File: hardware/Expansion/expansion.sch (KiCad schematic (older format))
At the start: 25 parts, among them J1 VID, J2 PPI, J3 PPO, P1 EXI, P2 EXO, U1 74LS138, U2 74LS00, U3 74LS123, U4 74LS20, U5 74LS175, U6 74LS245

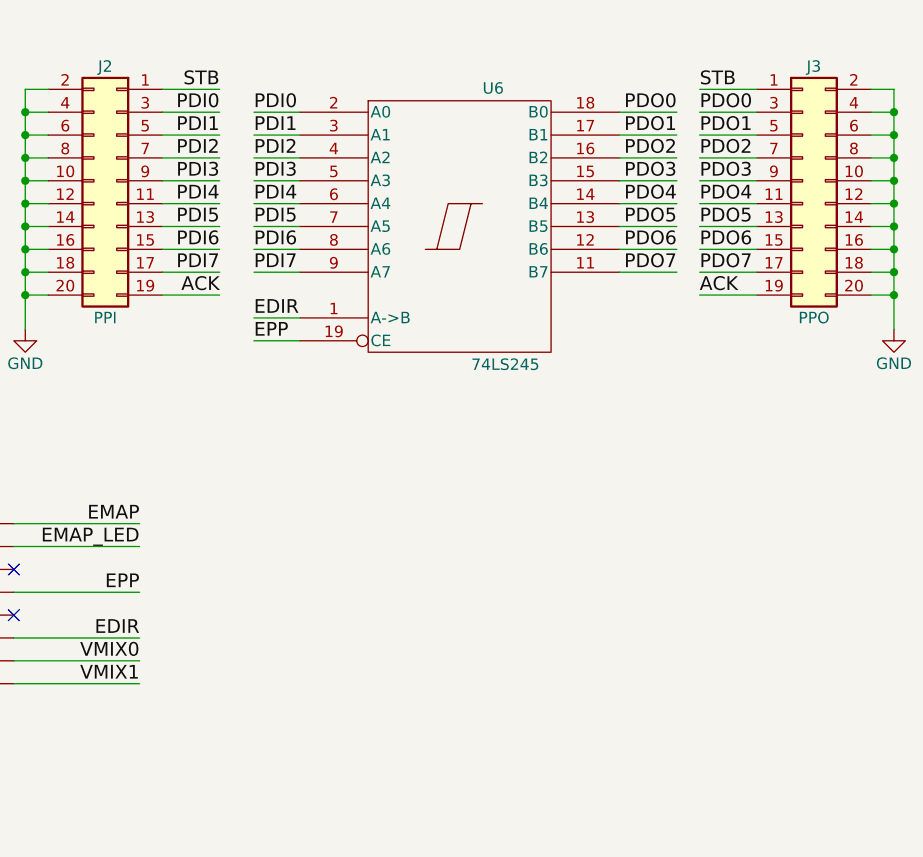
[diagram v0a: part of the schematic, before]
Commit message: revert:expansion
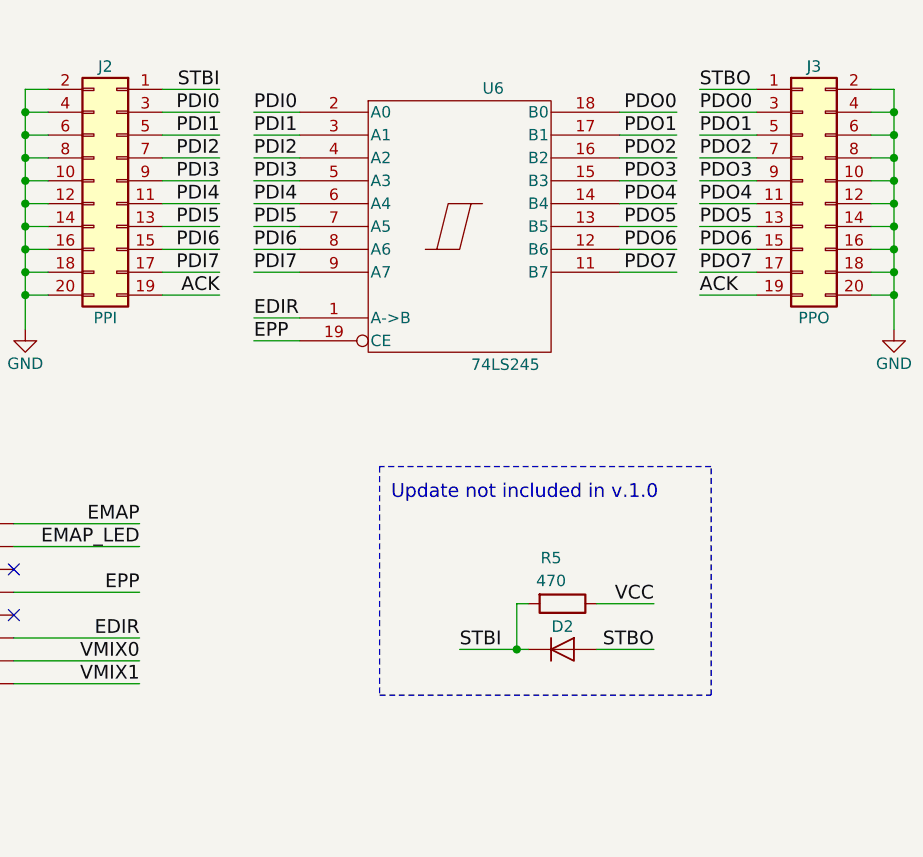
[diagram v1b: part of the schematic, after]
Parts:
- added D2: D, Diodes_THT:D_A-405_P7.62mm_Horizontal, symbol D
- added R5: 470, Resistors_THT:R_Axial_DIN0204_L3.6mm_D1.6mm_P7.62mm_Horizontal, symbol R
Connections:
- net VCC: now also R5.1
- net STB renamed STBI
- net STBI: now also D2.1 (K), R5.2; no longer J3.1 (Pin_1)
- new net STBO: D2.2 (A), J3.1 (Pin_1)
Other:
- note added: "Update not included in v.1.0"
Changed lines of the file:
@@
 Title "OricExos expansion board"
 Date "2018-11-30"
-Rev "1.0"
+Rev "1.1"
 Comp "copyright © 2018 iss"
 Comment1 ""
@@
 	7800 950  8050 950
 Text Label 8050 950  2    60   ~ 0
-STB
+STBI
 Wire Wire Line
 	10400 950  10150 950
 Text Label 10150 950  0    60   ~ 0
-STB
+STBO
 Wire Wire Line
 	10400 1850 10150 1850
@@
 	2550 3300 2550 4050
 Connection ~ 2550 4050
+$Comp
+L D D2
+U 1 1 5C12C7AE
+P 9550 3400
+F 0 "D2" H 9550 3500 50  0000 C CNN
+F 1 "D" H 9550 3300 50  0001 C CNN
+F 2 "Diodes_THT:D_A-405_P7.62mm_Horizontal" H 9550 3400 50  0001 C CNN
+F 3 "" H 9550 3400 50  0001 C CNN
+	1    9550 3400
+	1    0    0    -1
+$EndComp
+Wire Wire Line
+	9400 3400 9100 3400
+Text Label 9100 3400 0    60   ~ 0
+STBI
+Wire Wire Line
+	9700 3400 9950 3400
+Text Label 9950 3400 2    60   ~ 0
+STBO
+$Comp
+L R R5
+U 1 1 5C12D242
+P 9550 3200
+F 0 "R5" V 9350 3150 50  0000 C CNN
+F 1 "470" V 9450 3150 50  0000 C CNN
+F 2 "Resistors_THT:R_Axial_DIN0204_L3.6mm_D1.6mm_P7.62mm_Horizontal" V 9480 3200 50  0001 C CNN
+F 3 "" H 9550 3200 50  0001 C CNN
+	1    9550 3200
+	0    1    1    0
+$EndComp
+Wire Wire Line
+	9700 3200 9950 3200
+Text Label 9950 3200 2    60   ~ 0
+VCC
+Wire Wire Line
+	9400 3200 9350 3200
+Wire Wire Line
+	9350 3200 9350 3400
+Connection ~ 9350 3400
+Wire Notes Line
+	8750 2600 8750 3600
+Wire Notes Line
+	8750 3600 10200 3600
+Wire Notes Line
+	10200 3600 10200 2600
+Wire Notes Line
+	10200 2600 8750 2600
+Text Notes 8800 2750 0    60   ~ 0
+Update not included in v.1.0
 $EndSCHEMATC

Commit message: Revert "update:expansion"
This reverts commit fc7daa09fcab310e52193976a9df76314ecc8e0b.
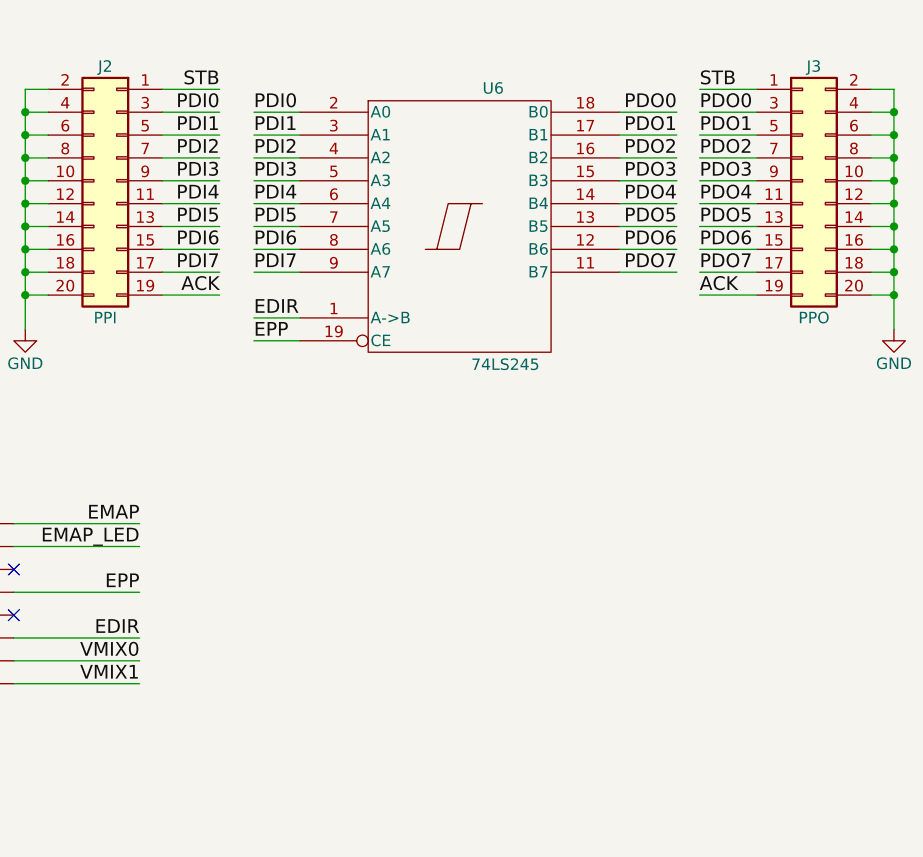
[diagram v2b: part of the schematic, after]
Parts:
- removed D2: D, Diodes_THT:D_A-405_P7.62mm_Horizontal, symbol D
- removed R5: 470, Resistors_THT:R_Axial_DIN0204_L3.6mm_D1.6mm_P7.62mm_Horizontal, symbol R
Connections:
- net STBO is gone; now on net STB: J3.1 (Pin_1)
- net STBI renamed STB
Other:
- note removed: "Update not included in v.1.0"
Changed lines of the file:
@@
 Title "OricExos expansion board"
 Date "2018-11-30"
-Rev "1.1"
+Rev "1.0"
 Comp "copyright © 2018 iss"
 Comment1 ""
@@
 	7800 950  8050 950
 Text Label 8050 950  2    60   ~ 0
-STBI
+STB
 Wire Wire Line
 	10400 950  10150 950
 Text Label 10150 950  0    60   ~ 0
-STBO
+STB
 Wire Wire Line
 	10400 1850 10150 1850
@@
 	2550 3300 2550 4050
 Connection ~ 2550 4050
-$Comp
-L D D2
-U 1 1 5C12C7AE
-P 9550 3400
-F 0 "D2" H 9550 3500 50  0000 C CNN
-F 1 "D" H 9550 3300 50  0001 C CNN
-F 2 "Diodes_THT:D_A-405_P7.62mm_Horizontal" H 9550 3400 50  0001 C CNN
-F 3 "" H 9550 3400 50  0001 C CNN
-	1    9550 3400
-	1    0    0    -1
-$EndComp
-Wire Wire Line
-	9400 3400 9100 3400
-Text Label 9100 3400 0    60   ~ 0
-STBI
-Wire Wire Line
-	9700 3400 9950 3400
-Text Label 9950 3400 2    60   ~ 0
-STBO
-$Comp
-L R R5
-U 1 1 5C12D242
-P 9550 3200
-F 0 "R5" V 9350 3150 50  0000 C CNN
-F 1 "470" V 9450 3150 50  0000 C CNN
-F 2 "Resistors_THT:R_Axial_DIN0204_L3.6mm_D1.6mm_P7.62mm_Horizontal" V 9480 3200 50  0001 C CNN
-F 3 "" H 9550 3200 50  0001 C CNN
-	1    9550 3200
-	0    1    1    0
-$EndComp
-Wire Wire Line
-	9700 3200 9950 3200
-Text Label 9950 3200 2    60   ~ 0
-VCC
-Wire Wire Line
-	9400 3200 9350 3200
-Wire Wire Line
-	9350 3200 9350 3400
-Connection ~ 9350 3400
-Wire Notes Line
-	8750 2600 8750 3600
-Wire Notes Line
-	8750 3600 10200 3600
-Wire Notes Line
-	10200 3600 10200 2600
-Wire Notes Line
-	10200 2600 8750 2600
-Text Notes 8800 2750 0    60   ~ 0
-Update not included in v.1.0
 $EndSCHEMATC
